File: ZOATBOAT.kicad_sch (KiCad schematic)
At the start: 130 parts, among them SW1 SW_Push_45deg, SW10 SW_Push_45deg, SW11 SW_Push_45deg, SW12 SW_Push_45deg, SW13 SW_Push_45deg, SW14 SW_Push_45deg, SW15 SW_Push_45deg, SW16 SW_Push_45deg, SW17 SW_Push_45deg, SW18 SW_Push_45deg, SW19 SW_Push_45deg, SW2 SW_Push_45deg, SW20 SW_Push_45deg, SW21 SW_Push_45deg, SW22 SW_Push_45deg, SW23 SW_Push_45deg, SW24 SW_Push_45deg, SW25 SW_Push_45deg, SW26 SW_Push_45deg, SW27 SW_Push_45deg, SW28 SW_Push_45deg, SW29 SW_Push_45deg, SW3 SW_Push_45deg, SW30 SW_Push_45deg, SW31 SW_Push_45deg, SW32 SW_Push_45deg, SW33 SW_Push_45deg, SW34 SW_Push_45deg, SW35 SW_Push_45deg, SW36 SW_Push_45deg, SW37 SW_Push_45deg, SW38 SW_Push_45deg, SW39 SW_Push_45deg, SW4 SW_Push_45deg, SW40 SW_Push_45deg, SW41 SW_Push_45deg, SW42 SW_Push_45deg, SW43 SW_Push_45deg, SW44 SW_Push_45deg, SW45 SW_Push_45deg, SW46 SW_Push_45deg, SW47 SW_Push_45deg, SW48 SW_Push_45deg, SW49 SW_Push_45deg, SW5 SW_Push_45deg, SW50 SW_Push_45deg, SW51 SW_Push_45deg, SW52 SW_Push_45deg, SW53 SW_Push_45deg, SW54 SW_Push_45deg, SW55 SW_Push_45deg, SW56 SW_Push_45deg, SW57 SW_Push_45deg, SW58 SW_Push_45deg, SW59 SW_Push_45deg, SW6 SW_Push_45deg, SW60 SW_Push_45deg, SW61 SW_Push_45deg, SW62 SW_Push_45deg, SW63 SW_Push_45deg, SW64 SW_Push_45deg, SW65 RotaryEncoder_Switch, SW66 RotaryEncoder_Switch, SW7 SW_Push_45deg, SW8 SW_Push_45deg, SW9 SW_Push_45deg

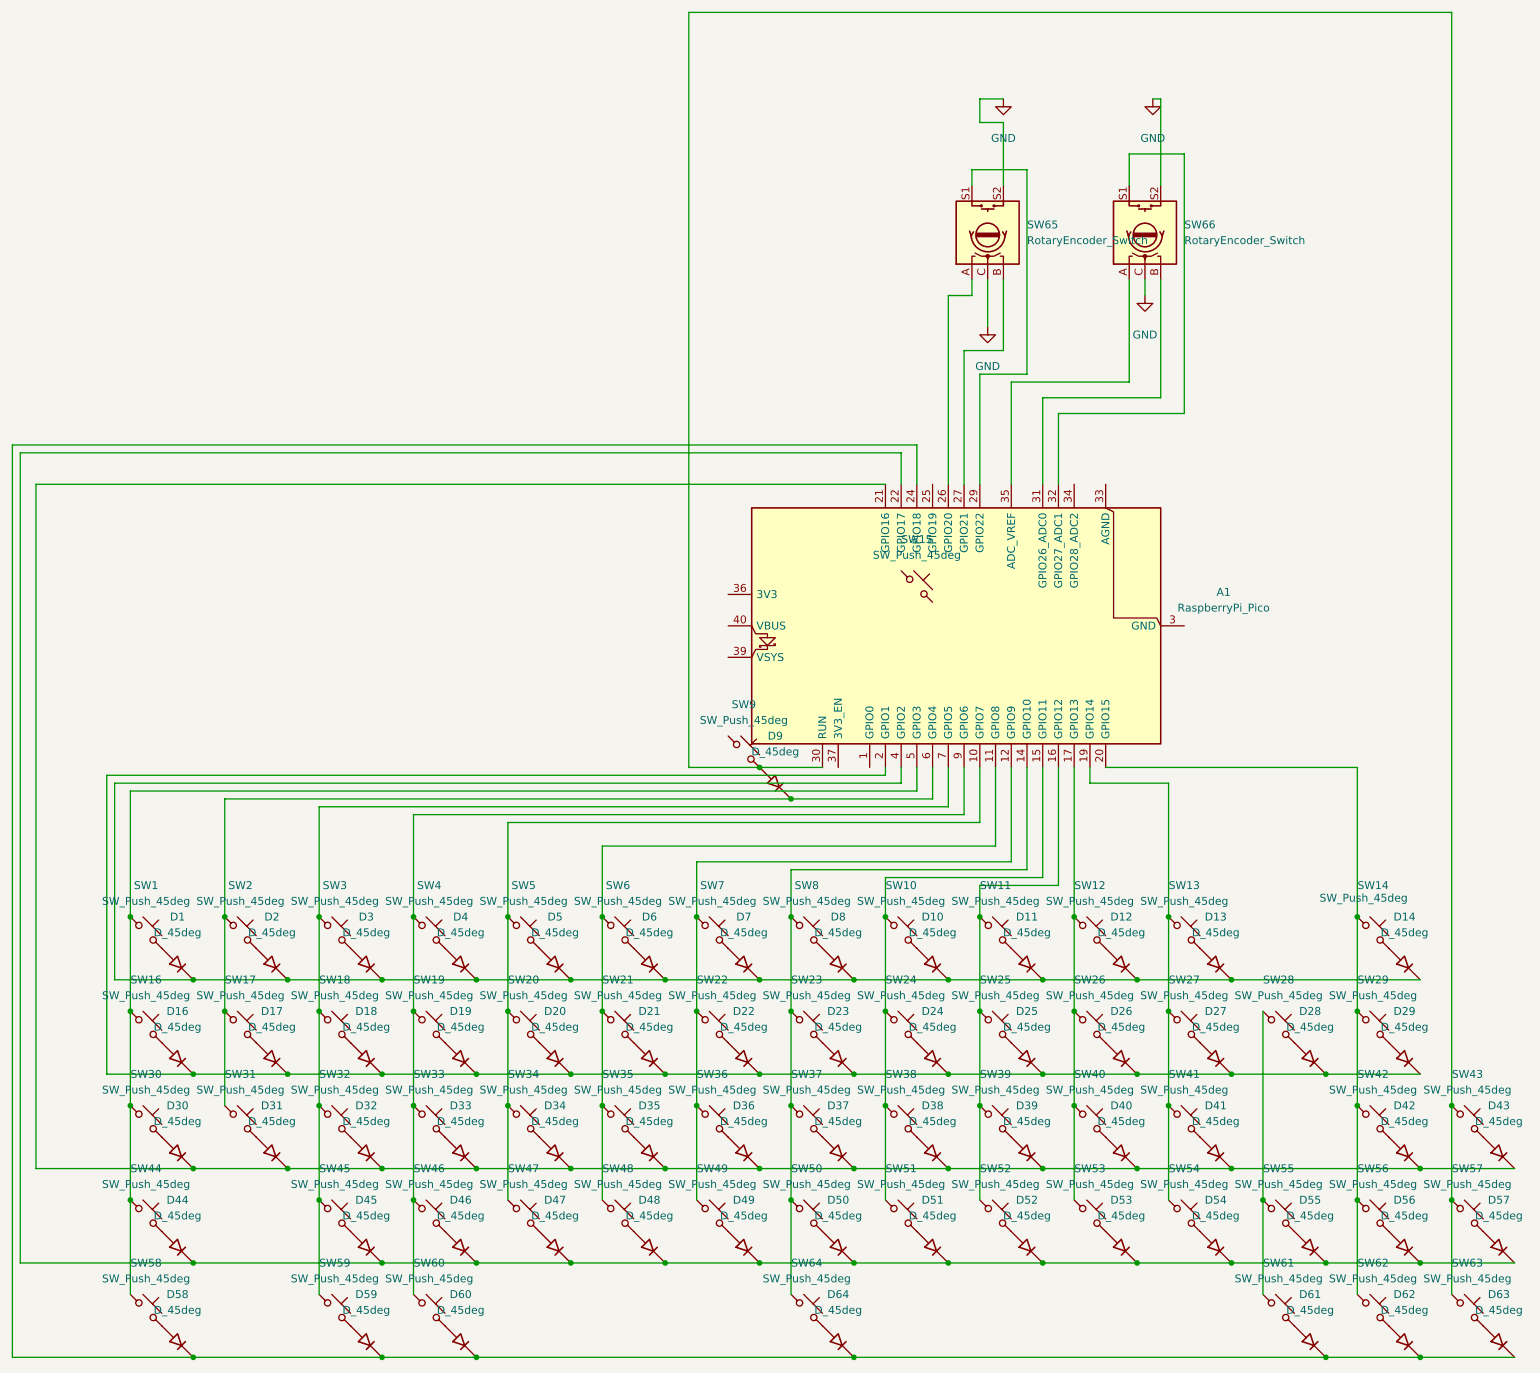
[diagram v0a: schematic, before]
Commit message: redid the wiring a fixed a couple of mistakes
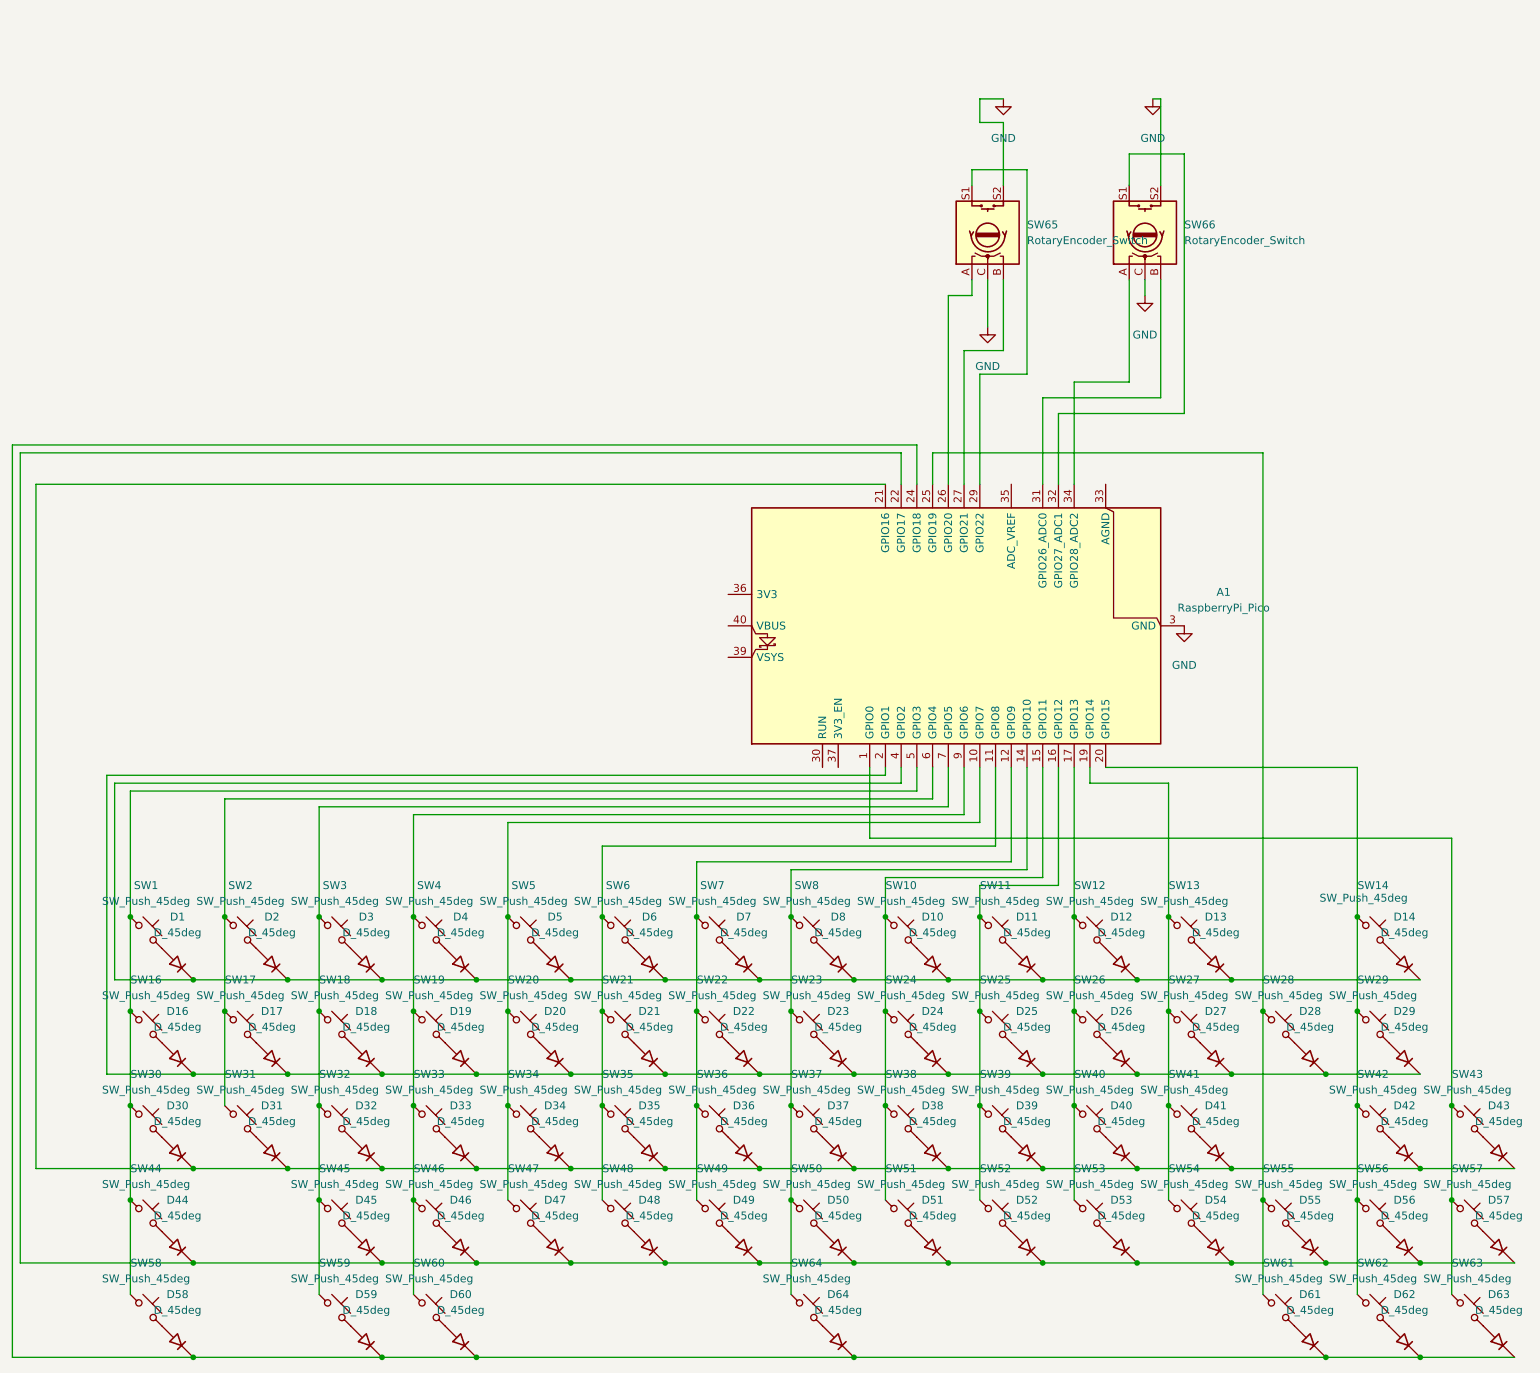
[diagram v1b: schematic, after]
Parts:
- removed D9: D_45deg, Diode_THT:D_A-405_P7.62mm_Horizontal, symbol Device:D_45deg
- removed SW15, SW9: SW_Push_45deg, ScottoKeebs_Hotswap:Hotswap_MX_1.00u, symbol Switch:SW_Push_45deg
- D64: footprint (none) -> Diode_THT:D_A-405_P7.62mm_Horizontal
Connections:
- net GND: now also A1.13 (GND), A1.18 (GND), A1.23 (GND), A1.28 (GND), A1.3 (GND), A1.38 (GND), A1.8 (GND)
- net at SW28.1, SW55.1, SW61.1: now also A1.25 (GPIO19)
- net at SW66.A: now also A1.34 (GPIO28_ADC2); no longer A1.35 (ADC_VREF)
- net at SW43.1, SW57.1, SW63.1: now also A1.1 (GPIO0); no longer A1.30 (RUN)
